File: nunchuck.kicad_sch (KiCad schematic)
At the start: 56 parts, among them J2 USB_C_Receptacle_USB2.0_14P, J3 USB_C_Receptacle_USB2.0_14P, SW1 BOOT, SW2 RESET, SW3 BOOT, SW4 RESET, U1 CH552T, U2 CH552T, U3 USBLC6-2SC6, U4 USBLC6-2SC6

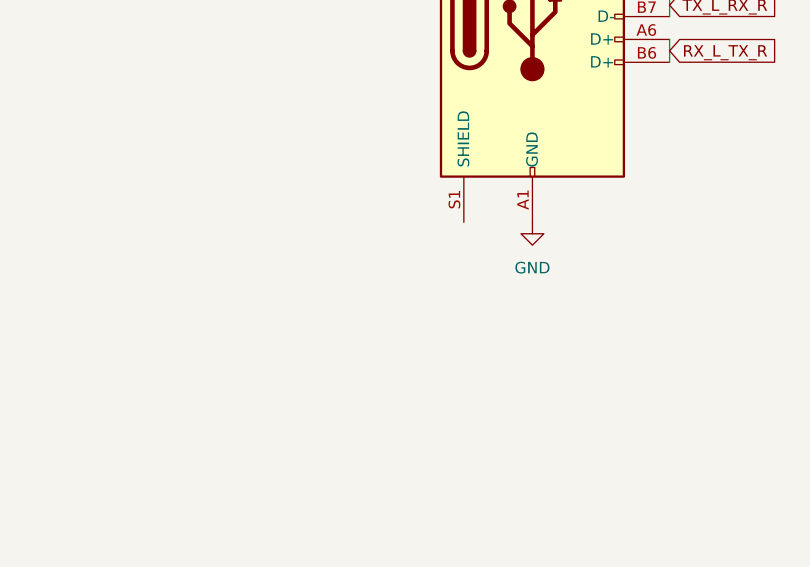
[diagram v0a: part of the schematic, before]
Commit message: before hexing
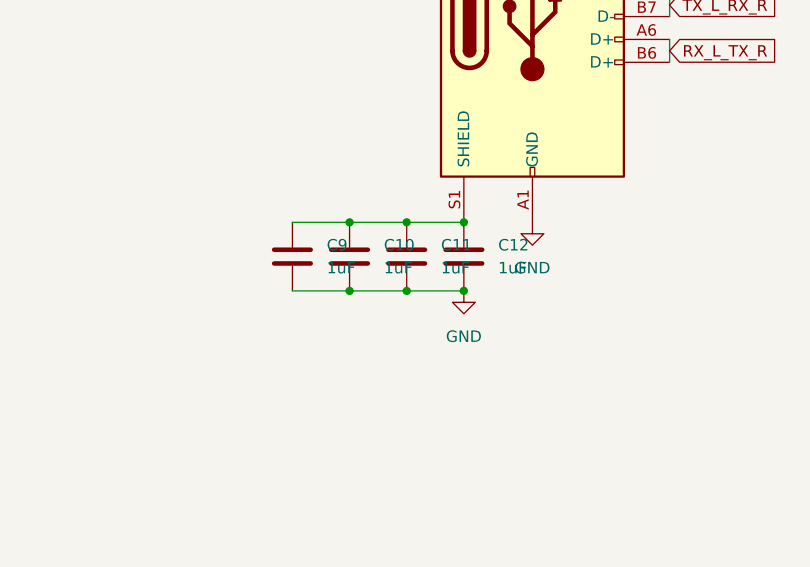
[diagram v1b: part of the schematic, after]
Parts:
- added C10, C11, C12, C9: 1uF, Capacitor_SMD:C_0603_1608Metric_Pad1.08x0.95mm_HandSolder, symbol Device:C
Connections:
- net GND: now also C10.2, C11.2, C12.2, C9.2
- net at J2.S1 (SHIELD): now also C10.1, C11.1, C12.1, C9.1
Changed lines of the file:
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@@
   (junction (at 53.34 44.45) (diameter 0) (color 0 0 0 0)
   )
+  (junction (at 233.045 152.4) (diameter 0) (color 0 0 0 0)
+  )
   (junction (at 99.06 26.67) (diameter 0) (color 0 0 0 0)
   )
@@
   (junction (at 53.34 31.75) (diameter 0) (color 0 0 0 0)
   )
+  (junction (at 233.045 160.02) (diameter 0) (color 0 0 0 0)
+  )
   (junction (at 137.16 67.31) (diameter 0) (color 0 0 0 0)
   )
@@
   (junction (at 143.51 74.93) (diameter 0) (color 0 0 0 0)
   )
+  (junction (at 226.695 152.4) (diameter 0) (color 0 0 0 0)
+  )
   (junction (at 88.9 31.75) (diameter 0) (color 0 0 0 0)
   )
+  (junction (at 220.345 152.4) (diameter 0) (color 0 0 0 0)
+  )
+  (junction (at 220.345 160.02) (diameter 0) (color 0 0 0 0)
+  )
   (junction (at 149.86 67.31) (diameter 0) (color 0 0 0 0)
   )
@@
   )
   (junction (at 172.72 36.83) (diameter 0) (color 0 0 0 0)
+  )
+  (junction (at 226.695 160.02) (diameter 0) (color 0 0 0 0)
   )
   (junction (at 76.2 29.21) (diameter 0) (color 0 0 0 0)
@@
     (stroke (width 0) (type default))
   )
+  (wire (pts (xy 213.995 160.02) (xy 220.345 160.02))
+    (stroke (width 0) (type default))
+  )
   (wire (pts (xy 255.905 125.73) (xy 266.065 125.73))
     (stroke (width 0) (type default))
@@
     (stroke (width 0) (type default))
   )
+  (wire (pts (xy 220.345 160.02) (xy 226.695 160.02))
+    (stroke (width 0) (type default))
+  )
   (wire (pts (xy 91.44 148.59) (xy 99.06 148.59))
     (stroke (width 0) (type default))
@@
     (stroke (width 0) (type default))
   )
+  (wire (pts (xy 220.345 152.4) (xy 226.695 152.4))
+    (stroke (width 0) (type default))
+  )
   (wire (pts (xy 172.72 41.91) (xy 172.72 44.45))
     (stroke (width 0) (type default))
@@
     (stroke (width 0) (type default))
   )
+  (wire (pts (xy 226.695 160.02) (xy 233.045 160.02))
+    (stroke (width 0) (type default))
+  )
   (wire (pts (xy 143.51 74.93) (xy 149.86 74.93))
     (stroke (width 0) (type default))
@@
     (stroke (width 0) (type default))
   )
+  (wire (pts (xy 226.695 152.4) (xy 233.045 152.4))
+    (stroke (width 0) (type default))
+  )
   (wire (pts (xy 111.76 41.91) (xy 119.38 41.91))
     (stroke (width 0) (type default))
@@
     (stroke (width 0) (type default))
   )
+  (wire (pts (xy 213.995 152.4) (xy 220.345 152.4))
+    (stroke (width 0) (type default))
+  )
   (wire (pts (xy 130.81 74.93) (xy 137.16 74.93))
     (stroke (width 0) (type default))
@@
     (property "Intersheetrefs" "${INTERSHEET_REFS}" (at 204.2667 35.56 0)
       (effects (font (size 1.27 1.27)) (justify right) hide)
+    )
+  )
+  (symbol (lib_id "Device:C") (at 233.045 156.21 0) (unit 1)
+    (in_bom yes) (on_board yes) (dnp no) (fields_autoplaced)
+    (property "Reference" "C12" (at 236.855 154.94 0)
+      (effects (font (size 1.27 1.27)) (justify left))
+    )
+    (property "Value" "1uF" (at 236.855 157.48 0)
+      (effects (font (size 1.27 1.27)) (justify left))
+    )
+    (property "Footprint" "Capacitor_SMD:C_0603_1608Metric_Pad1.08x0.95mm_HandSolder" (at 234.0102 160.02 0)
+      (effects (font (size 1.27 1.27)) hide)
+    )
+    (property "Datasheet" "~" (at 233.045 156.21 0)
+      (effects (font (size 1.27 1.27)) hide)
+    )
+    (pin "2")
+    (pin "1")
+    (instances
+      (project "nunchuck"
+        (path "/b46ad75c-c7a1-4bfe-a2f6-0c79981e5dbf"
+          (reference "C12") (unit 1)
+        )
+      )
+    )
+  )
+  (symbol (lib_id "power:GND") (at 233.045 160.02 0) (mirror y) (unit 1)
+    (in_bom yes) (on_board yes) (dnp no)
+    (property "Reference" "#PWR030" (at 233.045 166.37 0)
+      (effects (font (size 1.27 1.27)) hide)
+    )
+    (property "Value" "GND" (at 233.045 165.1 0)
+      (effects (font (size 1.27 1.27)))
+    )
+    (property "Footprint" "" (at 233.045 160.02 0)
+      (effects (font (size 1.27 1.27)) hide)
+    )
+    (property "Datasheet" "" (at 233.045 160.02 0)
+      (effects (font (size 1.27 1.27)) hide)
+    )
+    (pin "1")
+    (instances
+      (project "nunchuck"
+        (path "/b46ad75c-c7a1-4bfe-a2f6-0c79981e5dbf"
+          (reference "#PWR030") (unit 1)
+        )
+      )
     )
   )
@@
     )
   )
+  (symbol (lib_id "Device:C") (at 220.345 156.21 0) (unit 1)
+    (in_bom yes) (on_board yes) (dnp no) (fields_autoplaced)
+    (property "Reference" "C10" (at 224.155 154.94 0)
+      (effects (font (size 1.27 1.27)) (justify left))
+    )
+    (property "Value" "1uF" (at 224.155 157.48 0)
+      (effects (font (size 1.27 1.27)) (justify left))
+    )
+    (property "Footprint" "Capacitor_SMD:C_0603_1608Metric_Pad1.08x0.95mm_HandSolder" (at 221.3102 160.02 0)
+      (effects (font (size 1.27 1.27)) hide)
+    )
+    (property "Datasheet" "~" (at 220.345 156.21 0)
+      (effects (font (size 1.27 1.27)) hide)
+    )
+    (pin "2")
+    (pin "1")
+    (instances
+      (project "nunchuck"
+        (path "/b46ad75c-c7a1-4bfe-a2f6-0c79981e5dbf"
+          (reference "C10") (unit 1)
+        )
+      )
+    )
+  )
   (symbol (lib_id "Diode:BAV70") (at 76.2 21.59 0) (mirror y) (unit 1)
     (in_bom yes) (on_board yes) (dnp no)
@@
         (path "/b46ad75c-c7a1-4bfe-a2f6-0c79981e5dbf"
           (reference "#PWR016") (unit 1)
+        )
+      )
+    )
+  )
+  (symbol (lib_id "Device:C") (at 226.695 156.21 0) (unit 1)
+    (in_bom yes) (on_board yes) (dnp no) (fields_autoplaced)
+    (property "Reference" "C11" (at 230.505 154.94 0)
+      (effects (font (size 1.27 1.27)) (justify left))
+    )
+    (property "Value" "1uF" (at 230.505 157.48 0)
+      (effects (font (size 1.27 1.27)) (justify left))
+    )
+    (property "Footprint" "Capacitor_SMD:C_0603_1608Metric_Pad1.08x0.95mm_HandSolder" (at 227.6602 160.02 0)
+      (effects (font (size 1.27 1.27)) hide)
+    )
+    (property "Datasheet" "~" (at 226.695 156.21 0)
+      (effects (font (size 1.27 1.27)) hide)
+    )
+    (pin "2")
+    (pin "1")
+    (instances
+      (project "nunchuck"
+        (path "/b46ad75c-c7a1-4bfe-a2f6-0c79981e5dbf"
+          (reference "C11") (unit 1)
         )
       )
@@
         )
       )
+    )
+  )
+  (symbol (lib_id "Device:C") (at 213.995 156.21 0) (unit 1)
+    (in_bom yes) (on_board yes) (dnp no) (fields_autoplaced)
+    (property "Reference" "C9" (at 217.805 154.94 0)
+      (effects (font (size 1.27 1.27)) (justify left))
+    )
+    (property "Value" "1uF" (at 217.805 157.48 0)
+      (effects (font (size 1.27 1.27)) (justify left))
+    )
+    (property "Footprint" "Capacitor_SMD:C_0603_1608Metric_Pad1.08x0.95mm_HandSolder" (at 214.9602 160.02 0)
+      (effects (font (size 1.27 1.27)) hide)
+    )
+    (property "Datasheet" "~" (at 213.995 156.21 0)
+      (effects (font (size 1.27 1.27)) hide)
+    )
+    (pin "2")
+    (pin "1")
+    (instances
+      (project "nunchuck"
+        (path "/b46ad75c-c7a1-4bfe-a2f6-0c79981e5dbf"
+          (reference "C9") (unit 1)
+        )
+      )
